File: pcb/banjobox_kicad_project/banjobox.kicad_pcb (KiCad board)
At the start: 2 copper layers, 20 parts, among them SW1 RotaryEncoder_Switch, U1 SHT31-DIS, U2 ER_OLEDM0.91_1x-I2C, U3 LM1117T-3.3, U4 MOUDLE-SEEEDUINO-XIAO, U5 PAM8302AAD

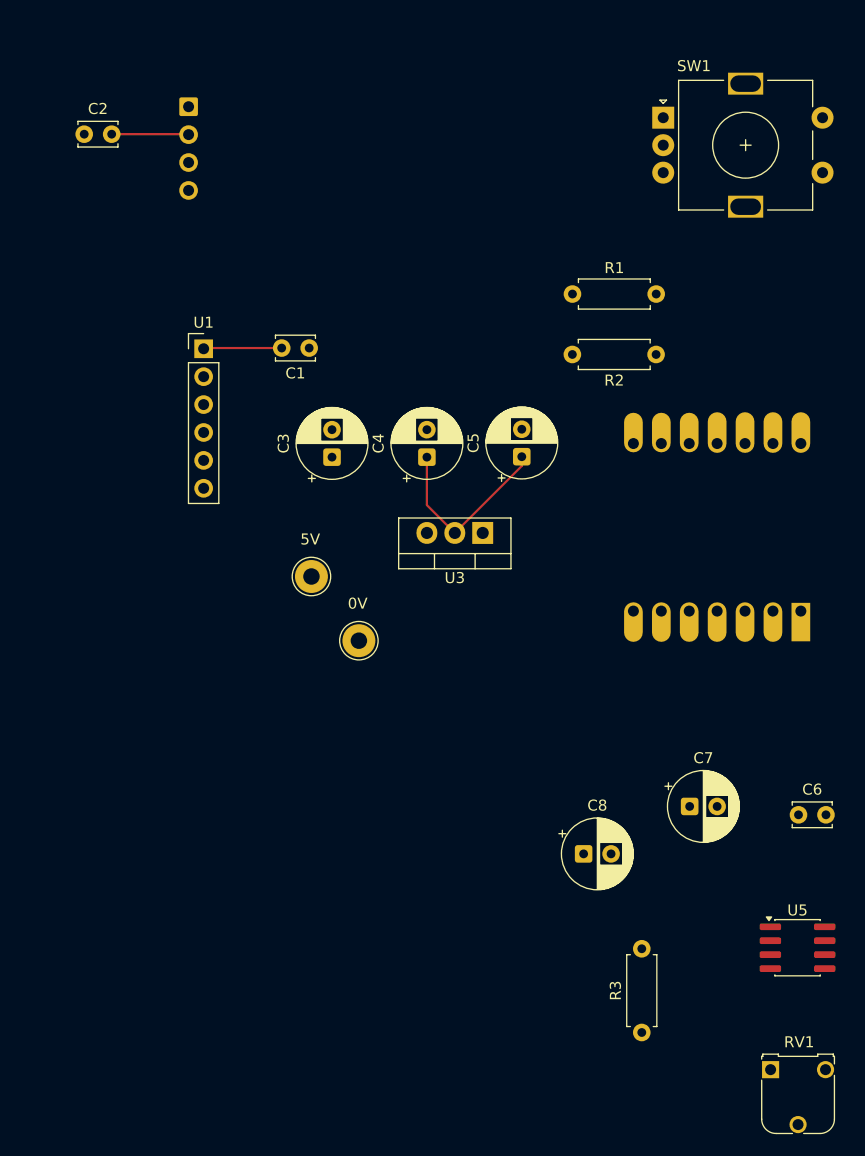
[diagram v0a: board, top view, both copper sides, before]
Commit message: forgot to save after last commit, routed pcb
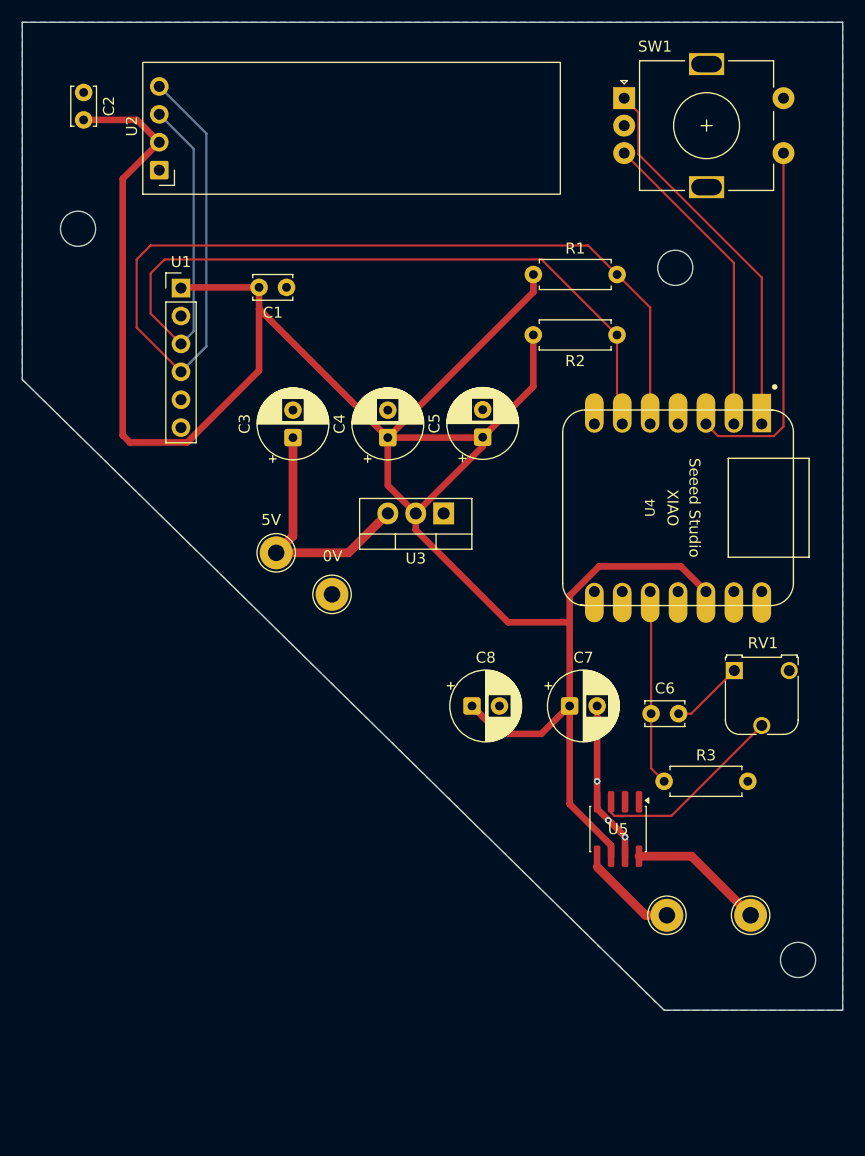
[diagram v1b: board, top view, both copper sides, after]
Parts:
- removed the REF** at (117.0, 101.5)
- removed the REF** at (112.7, 95.7)
- added REF**: MountingHole_3.2mm_M3, MountingHole:MountingHole_3.2mm_M3, F.Cu at (91.4, 64.0)
- added REF**: MountingHole_3.2mm_M3, MountingHole:MountingHole_3.2mm_M3, F.Cu at (157.0, 130.6)
- added REF**: MountingHole_3.2mm_M3, MountingHole:MountingHole_3.2mm_M3, F.Cu at (145.8, 67.6)
- added TP1: TestPoint, TestPoint:TestPoint_THTPad_D3.0mm_Drill1.5mm, F.Cu at (109.5, 93.5)
- added TP2: TestPoint, TestPoint:TestPoint_THTPad_D3.0mm_Drill1.5mm, F.Cu at (114.6, 97.3)
- added TP3: TestPoint, TestPoint:TestPoint_THTPad_D3.0mm_Drill1.5mm, F.Cu at (145.0, 126.5)
- added TP4: TestPoint, TestPoint:TestPoint_THTPad_D3.0mm_Drill1.5mm, F.Cu at (152.7, 126.5)
- U2, U4: moved to F.Cu
- moved RV1 36.5 mm to (151.2, 104.2)
- moved R3 23.0 mm to (144.8, 114.3), turned to 0 degrees
- moved U5 19.6 mm to (140.6, 118.6), turned to -90 degrees
- moved C8 16.9 mm to (127.3, 107.4)
- moved C6 16.3 mm to (143.6, 108.1)
- moved C7 14.2 mm to (136.2, 107.4)
- moved U2 6.36 mm to (98.8, 58.7), turned to 90 degrees
- moved U1 5.90 mm to (100.8, 69.4)
- moved C1 5.90 mm to (110.4, 69.3)
- moved R1 3.98 mm to (132.9, 68.2)
- moved R2 3.98 mm to (140.5, 73.7)
- moved U3 3.98 mm to (124.7, 89.9)
- moved C3 3.98 mm to (111.0, 83.0)
- moved C4 3.98 mm to (119.6, 83.0)
- moved C5 3.98 mm to (128.3, 83.0)
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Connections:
- net +5V renamed +BATT
- net GND renamed -BATT
- U4 pad 10: unconnected-(U4-PA5_A9_D9_MISO-Pad10) -> PWM
- U4 pad 4: PWM -> unconnected-(U4-PA11_A3_D3-Pad4)
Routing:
- net VCC: track 31.6 -> 209.8 mm
- net SDA: track 0.00 -> 100.8 mm
- net SCL: track 0.00 -> 84.3 mm
- net EC11A: track 0.00 -> 34.8 mm
- net EC11SW1: track 0.00 -> 32.8 mm
- net EC11B: track 0.00 -> 28.8 mm
- net +BATT: track 0.00 -> 22.8 mm
- net Net-(U5-IN+): track 0.00 -> 18.2 mm
- net PWM: track 0.00 -> 17.8 mm
- net -BATT: track 0.00 -> 15.1 mm, vias 0 -> 4
- net Net-(U5-OUT-): track 0.00 -> 12.4 mm
- net Net-(U5-OUT+): track 0.00 -> 9.15 mm
- net Net-(C6-Pad2): track 0.00 -> 6.70 mm
- added copper zone on B.Cu, net -BATT
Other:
- board outline added: 74.7 x 89.9 mm
